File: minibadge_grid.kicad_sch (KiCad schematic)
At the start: 16 parts, among them J1 Board to Board

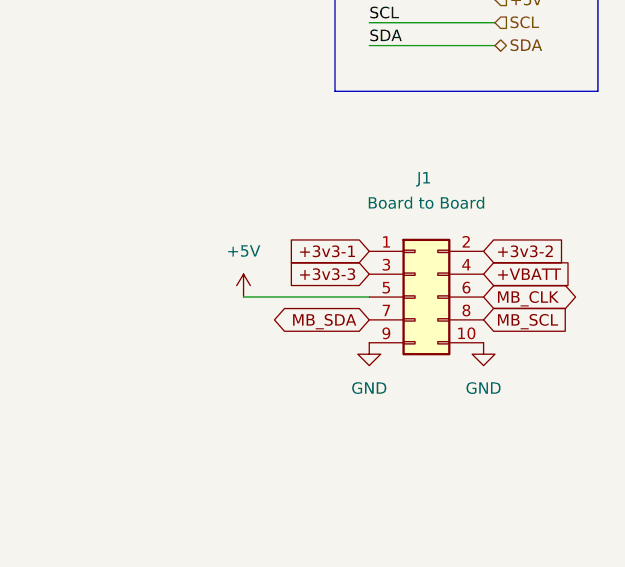
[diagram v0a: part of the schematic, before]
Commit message: cleanup
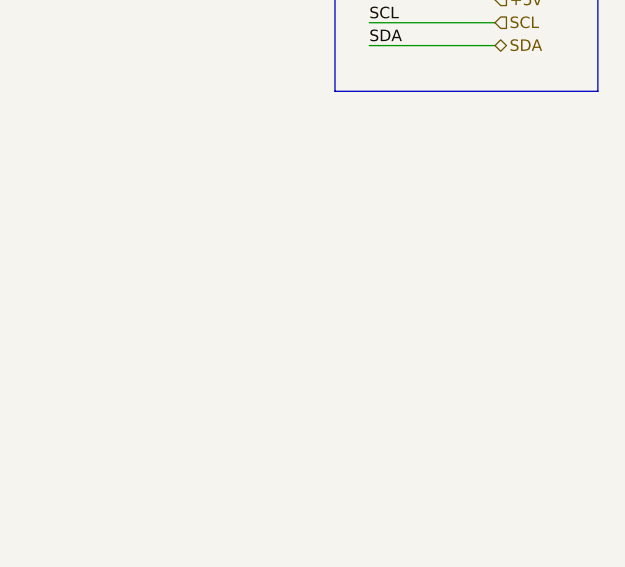
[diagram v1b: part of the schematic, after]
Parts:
- removed J1: Board to Board, symbol Connector_Generic:Conn_02x05_Odd_Even
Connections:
- net +VBATT renamed +5v
